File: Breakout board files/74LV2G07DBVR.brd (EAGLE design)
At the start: 20.2 x 15.1 mm, 7 parts, among them IC1 SN74LVC2G07DBVR

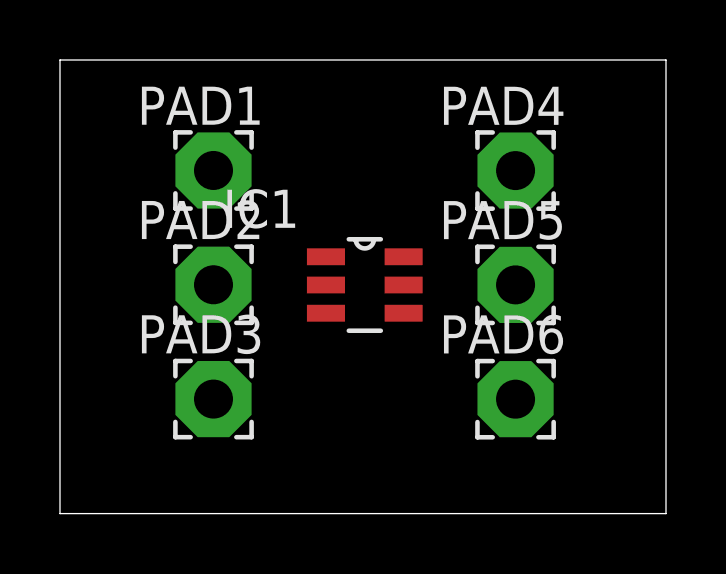
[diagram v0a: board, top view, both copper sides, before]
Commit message: Breakout Board Solutions
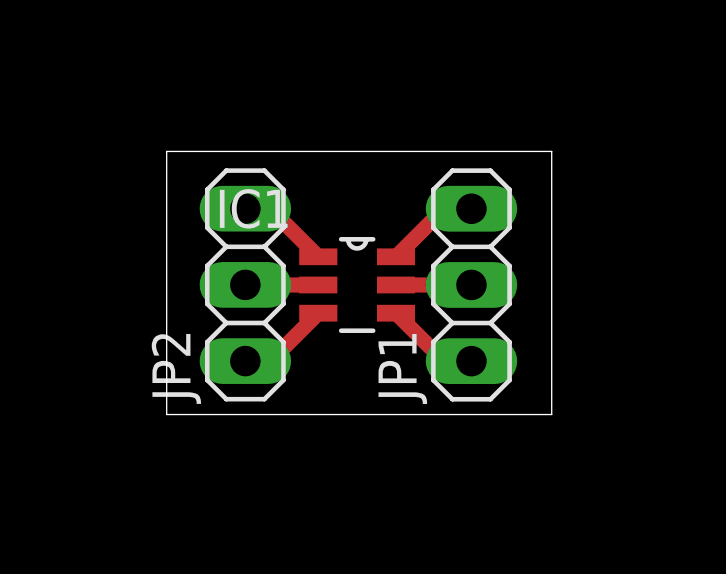
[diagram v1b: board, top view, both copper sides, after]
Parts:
- removed PAD1, PAD2, PAD3, PAD4, PAD5, PAD6: (no value), ee2parts:2,54/1,1
- added JP1, JP2: (no value), pinhead:1X03
- moved IC1 0.25 mm to (9.91, 7.62)
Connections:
- net N$1: now also JP2.2; no longer PAD2.1
- net N$2: now also JP2.3; no longer PAD1.1
- net N$3: now also JP2.1; no longer PAD3.1
- net N$4: now also JP1.3; no longer PAD4.1
- net N$5: now also JP1.1; no longer PAD6.1
- net N$6: now also JP1.2; no longer PAD5.1
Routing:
- net N$4: track 0.00 -> 3.18 mm
- net N$5: track 0.00 -> 3.18 mm
- net N$2: track 0.00 -> 3.10 mm
- net N$3: track 0.00 -> 3.09 mm
- net N$6: track 0.00 -> 2.51 mm
- net N$1: track 0.00 -> 2.43 mm
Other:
- board size 20.2 x 15.1 mm -> 12.8 x 8.8 mm
